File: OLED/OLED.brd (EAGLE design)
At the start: 35.6 x 29.8 mm, 25 parts

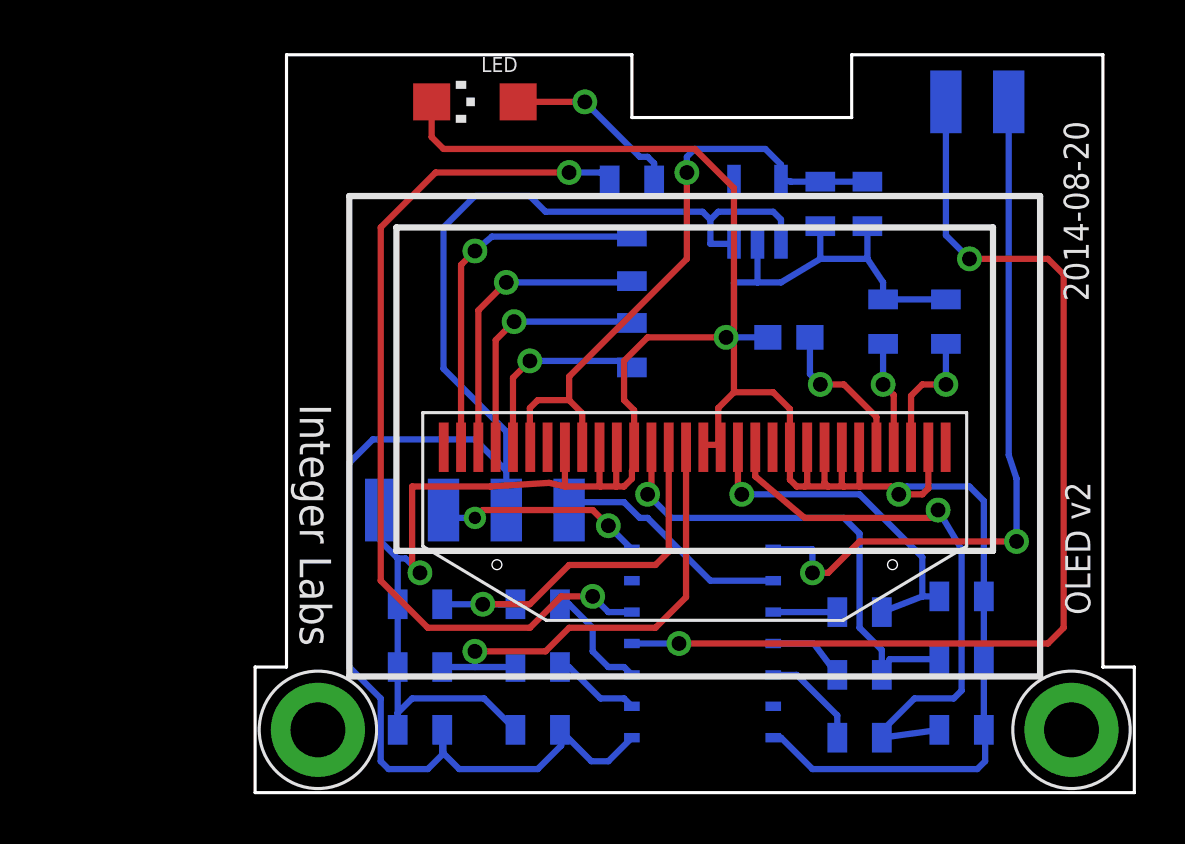
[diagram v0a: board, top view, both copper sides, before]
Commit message: minor revisions
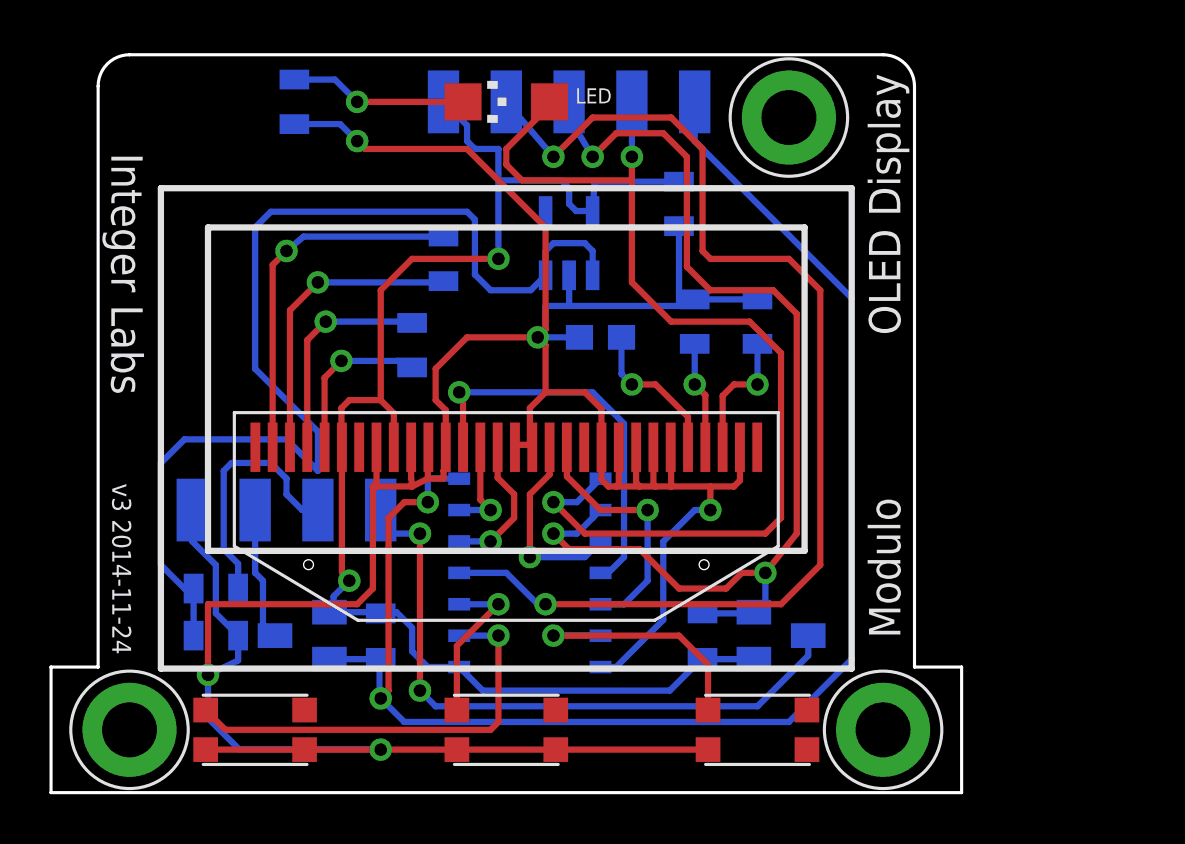
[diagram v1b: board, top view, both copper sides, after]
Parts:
- removed C1, C9: 0.1uF, SparkFun-Capacitors:0805
- removed R10, R4, R6, R8: 2k, SparkFun-Resistors:0805
- removed R11, R3, R5, R7, R9: 1k, SparkFun-Resistors:0805
- added Q1, Q2: MOSFET-NCHANNELBSS138, SparkFun-DiscreteSemi:SOT23
- added R13, R14: 2k, SparkFun-Passives:0805
- added U$4: FOOTPRINTFOOTPRINT-2, IntegerLabs:FOOTPRINT2
- added U$6, U$7: TACT-SWITCHKMR2, IntegerLabs:TACT-SWITCH-SMALL
- C10, C2: value 10uF -> .47uF
- R2: value 2k -> 1; device SparkFun-Resistors:0805 -> SparkFun-Passives:0805
- U$5: value FOOTPRINTFOOTPRINT-2 -> TACT-SWITCHKMR2; device IntegerLabs:FOOTPRINT2 -> IntegerLabs:TACT-SWITCH-SMALL
- moved R12 14.0 mm to (9.21, 27.9), turned to 90 degrees
- moved C10 9.09 mm to (6.03, 6.35), turned to 0 degrees
- moved C5 8.89 mm to (14.0, 18.1)
- moved R2 8.28 mm to (6.03, 8.26)
- moved U$2 7.73 mm to (20.3, 22.2)
- moved C4 7.62 mm to (25.4, 19.1)
- moved C3 7.62 mm to (27.9, 19.1)
- moved R1 7.62 mm to (21.6, 18.4)
- moved C6 7.62 mm to (15.2, 21.6)
- moved C2 7.62 mm to (24.8, 23.8)
- moved U$1 7.62 mm to (17.8, 11.4)
- moved U$3 7.55 mm to (19.1, 5.08)
- moved U$5 2.54 mm to (7.62, 2.54)
- moved LED 1.27 mm to (17.8, 27.9)
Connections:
- removed net BUS_CLK: U$3.9, U$5.SCL
- removed net BUS_DATA: U$3.7, U$5.SDA
- removed net CS: R5.2, U$3.11
- removed net D/C: R7.2, U$3.2
- removed net LED: R12.2, U$3.5
- removed net MOSI: R11.2, U$3.12
- removed net N$13: R6.2, R7.1, U$1.15
- removed net N$14: R4.2, R5.1, U$1.13
- removed net N$15: R2.2, R3.1, U$1.14
- removed net N$5: LED.A, R12.1
- removed net N$8: R8.2, R9.1, U$1.18
- removed net PGM_MISO: U$3.8, U$5.MISO
- removed net PGM_RESET: U$3.4, U$5.RESET
- removed net SCK: R9.2, U$3.10
- new net BUTTON1: U$3.2, U$5.P1
- new net BUTTON2: U$3.3, U$6.P1
- new net BUTTON3: U$3.13, U$7.P1
- new net DISPLAY_CS: U$1.13, U$3.11
- new net DISPLAY_D/C: U$1.15, U$3.5
- new net DISPLAY_MOSI: U$1.19, U$3.12
- new net DISPLAY_RESET: U$1.14, U$3.6
- new net DISPLAY_SCK: U$1.18, U$3.10
- new net MISO/LED: LED.A, U$3.8, U$4.PROG3
- new net N$3: R2.2, U$4.BUS2
- new net SCL3.3/SCK: Q2.2, R14.1, U$3.9, U$4.PROG2
- new net SCL5: Q2.3, U$4.BUS3
- new net SDA3.3/MOSI: Q1.2, R13.1, U$3.7, U$4.PROG4
- new net SDA5: Q1.3, U$4.BUS1
- net +3.3V: now also Q1.1, Q2.1, R13.2, R14.2, U$3.1, U$4.PROG0; no longer C1.2
- net +5V: now also R2.1; no longer C9.2, U$3.1, U$5.VCC
- net GND: now also R12.1, U$4.BUS0, U$5.N1, U$5.N2, U$6.N1, U$6.N2, U$7.N1; no longer C1.1, C9.1, LED.C, R10.1, R2.1, R4.1, R6.1, R8.1, U$5.GND
- net N$7: now also LED.C, R12.2; no longer R10.2, R11.1, U$1.19
- net RESET: now also U$3.4, U$4.PROG1; no longer R3.2, U$3.3
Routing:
- net SDA3.3/MOSI: track 0.00 -> 60.9 mm, vias 0 -> 2
- net SCL3.3/SCK: track 0.00 -> 44.7 mm, vias 0 -> 3
- net PGM_RESET: track 42.8 -> 0.00 mm, vias 2 -> 0
- net MISO/LED: track 0.00 -> 42.1 mm, vias 0 -> 2
- net RESET: track 4.65 -> 46.6 mm, vias 0 -> 2
- net LED: track 36.3 -> 0.00 mm, vias 2 -> 0
- net +3.3V: track 25.6 -> 59.1 mm, vias 1 -> 2
- net PGM_MISO: track 29.2 -> 0.00 mm, vias 2 -> 0
- net SCL5: track 0.00 -> 26.5 mm, vias 0 -> 2
- net N$14: track 20.0 -> 0.00 mm, vias 1 -> 0
- net +5V: track 64.9 -> 44.9 mm
- net N$13: track 19.1 -> 0.00 mm, vias 1 -> 0
- net BUTTON1: track 0.00 -> 17.4 mm, vias 0 -> 1
- net DISPLAY_CS: track 0.00 -> 16.4 mm, vias 0 -> 1
- net N$15: track 16.3 -> 0.00 mm, vias 1 -> 0
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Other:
- board size 35.6 x 29.8 mm -> 36.8 x 29.8 mm
- board text added: "Modulo"
- board text added: "OLED Display"
- board text added: "v3 2014-11-24"
- board text removed: "2014-08-20"
- board text removed: "OLED v2"

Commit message: Checkpointing PCB designs
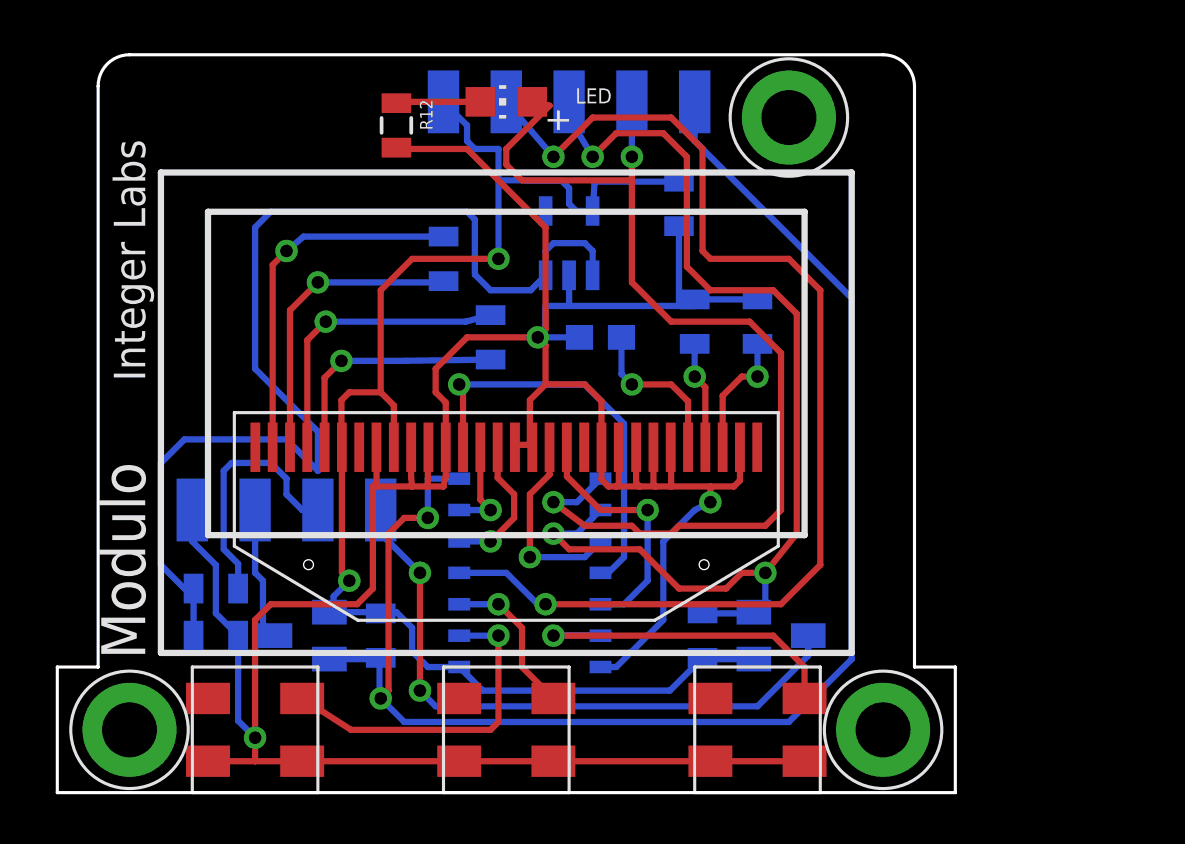
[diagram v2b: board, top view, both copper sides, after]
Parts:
- LED: device led:CHIPLED_1206 -> adafruit:CHIP-LED0805
- U$5, U$6, U$7: value TACT-SWITCHKMR2 -> TACT-SWITCHBOURNS-7914J; device IntegerLabs:TACT-SWITCH-SMALL -> IntegerLabs:BOURNS-7914J
- moved R12 4.24 mm to (13.3, 27.0), flipped to the top
- moved C5 3.19 mm to (17.1, 18.4)
- turned U$5 to 270 degrees
- turned U$6 to 270 degrees
- turned U$7 to 270 degrees
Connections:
- net BUTTON1: now also U$5.POS$1; no longer U$5.P1
- net BUTTON2: now also U$6.POS$1; no longer U$6.P1
- net BUTTON3: now also U$7.POS$1; no longer U$7.P1
- net GND: now also U$5.NEG$1, U$5.NEG$2, U$6.NEG$1, U$6.NEG$2, U$7.NEG$1, U$7.NEG$2; no longer U$5.N1, U$5.N2, U$6.N1, U$6.N2, U$7.N1
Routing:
- net GND: track 136.1 -> 129.7 mm, vias 5 -> 3
- net BUTTON1: track 17.4 -> 13.5 mm
- net N$7: track 7.20 -> 3.52 mm, vias 1 -> 0
- net BUTTON3: track 10.5 -> 13.9 mm
- net N$9: track 8.89 -> 12.1 mm
- net N$11: track 6.69 -> 9.81 mm
- net SCL5: track 26.5 -> 25.6 mm
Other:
- board size 36.8 x 29.8 mm -> 36.3 x 29.8 mm
- board text removed: "Integer Labs"
- board text removed: "Modulo"
- board text removed: "OLED Display"
- board text removed: "v3 2014-11-24"
